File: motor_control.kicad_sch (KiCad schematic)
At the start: 109 parts, among them J1 Conn_01x18_Pin, J2 Conn_01x18_Pin, J3 Conn_01x10_Pin

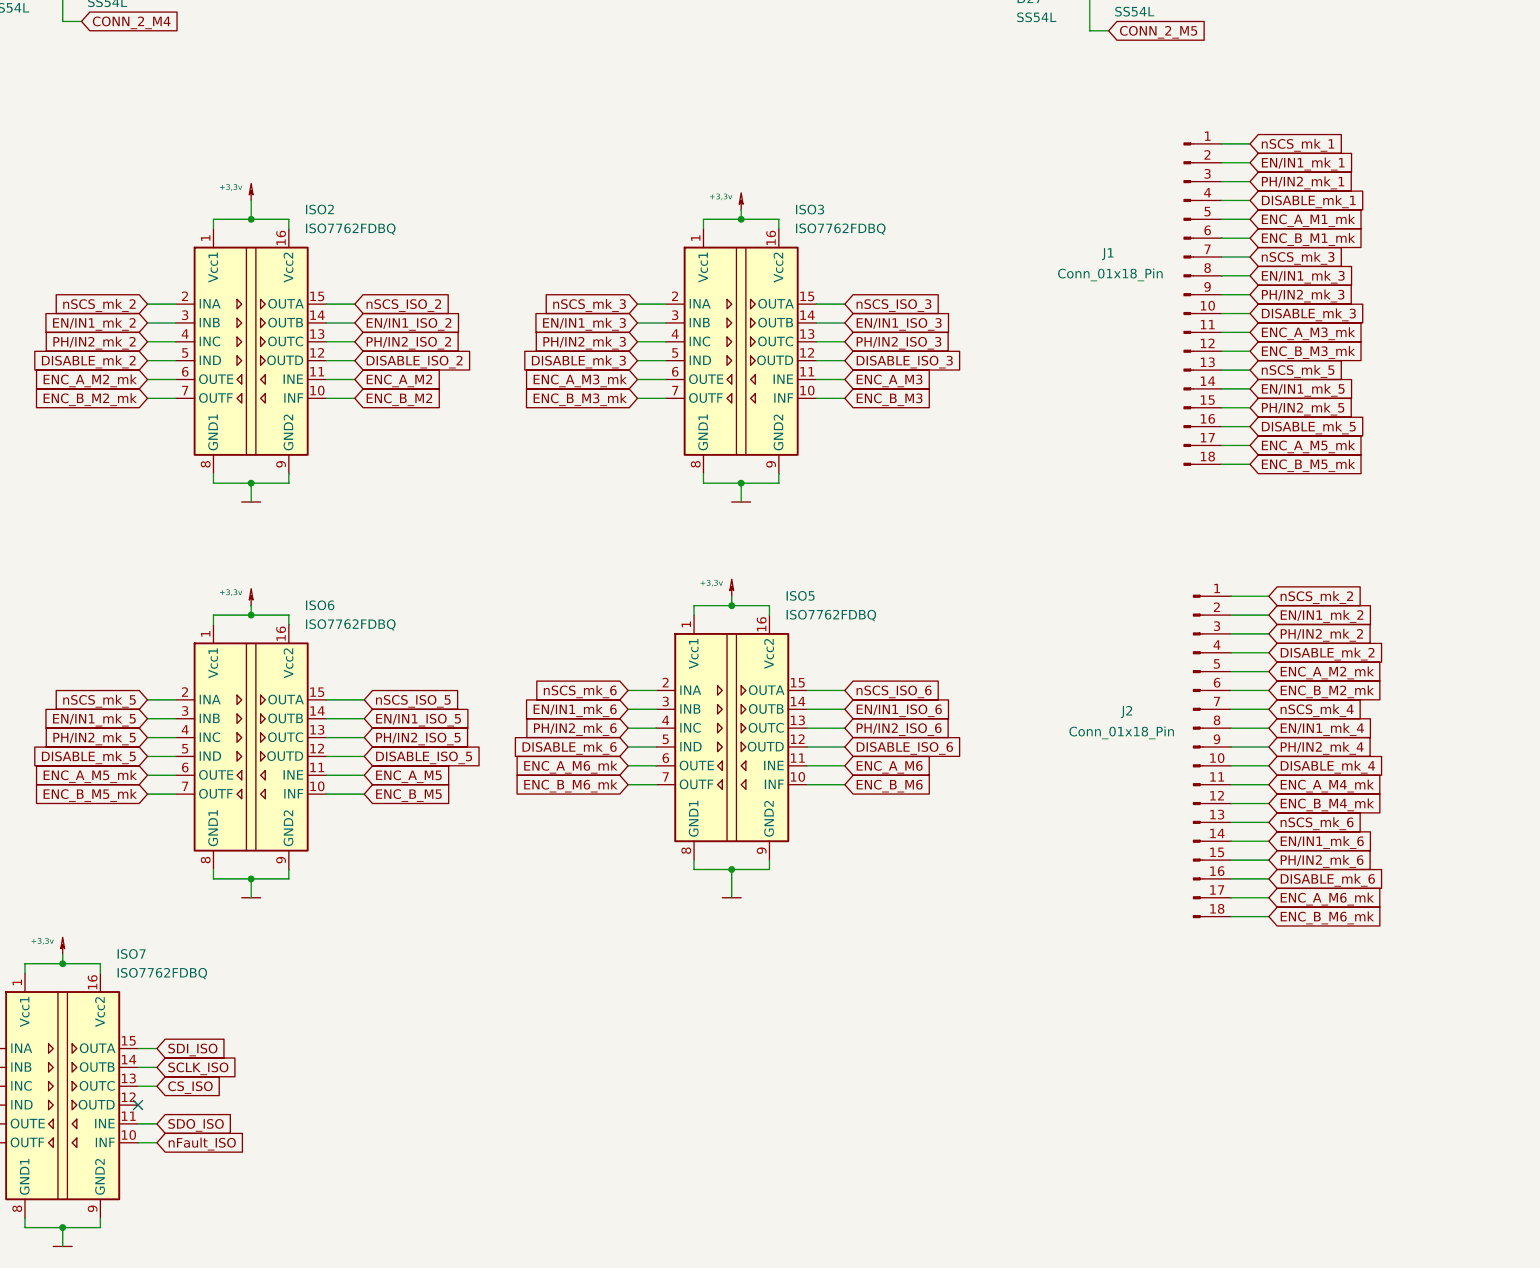
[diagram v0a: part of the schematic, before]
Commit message: I2C
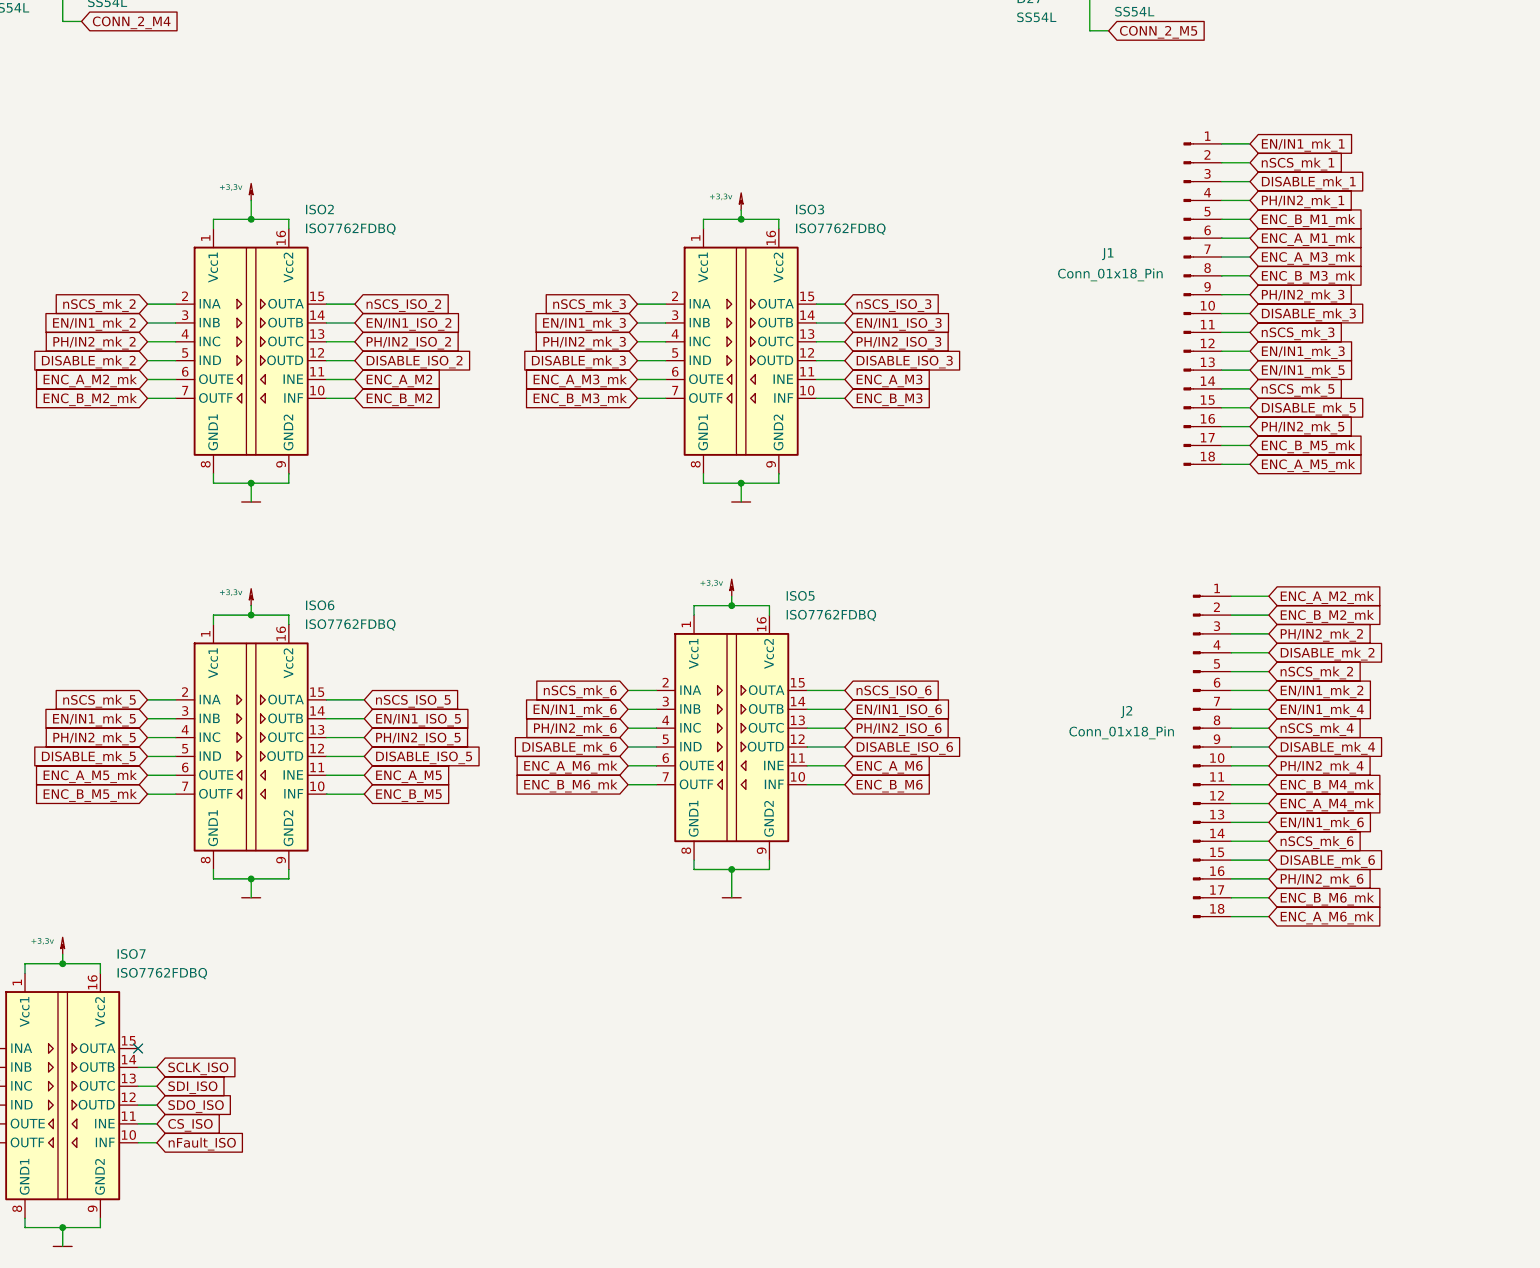
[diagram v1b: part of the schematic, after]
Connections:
- net CS_ISO: now also ISO7.11 (INE); no longer ISO7.13 (OUTC)
- net DISABLE_mk_1: now also J1.3 (Pin_3); no longer J1.4 (Pin_4)
- net DISABLE_mk_4: now also J2.9 (Pin_9); no longer J2.10 (Pin_10)
- net DISABLE_mk_5: now also J1.15 (Pin_15); no longer J1.16 (Pin_16)
- net DISABLE_mk_6: now also J2.15 (Pin_15); no longer J2.16 (Pin_16)
- net ENC_A_M1_mk: now also J1.6 (Pin_6); no longer J1.5 (Pin_5)
- net ENC_A_M2_mk: now also J2.1 (Pin_1); no longer J2.5 (Pin_5)
- net ENC_A_M3_mk: now also J1.7 (Pin_7); no longer J1.11 (Pin_11)
- net ENC_A_M4_mk: now also J2.12 (Pin_12); no longer J2.11 (Pin_11)
- net ENC_A_M5_mk: now also J1.18 (Pin_18); no longer J1.17 (Pin_17)
- net ENC_A_M6_mk: now also J2.18 (Pin_18); no longer J2.17 (Pin_17)
- net ENC_B_M1_mk: now also J1.5 (Pin_5); no longer J1.6 (Pin_6)
- net ENC_B_M2_mk: now also J2.2 (Pin_2); no longer J2.6 (Pin_6)
- net ENC_B_M3_mk: now also J1.8 (Pin_8); no longer J1.12 (Pin_12)
- net ENC_B_M4_mk: now also J2.11 (Pin_11); no longer J2.12 (Pin_12)
- net ENC_B_M5_mk: now also J1.17 (Pin_17); no longer J1.18 (Pin_18)
- net ENC_B_M6_mk: now also J2.17 (Pin_17); no longer J2.18 (Pin_18)
- net EN/IN1_mk_1: now also J1.1 (Pin_1); no longer J1.2 (Pin_2)
- net EN/IN1_mk_2: now also J2.6 (Pin_6); no longer J2.2 (Pin_2)
- net EN/IN1_mk_3: now also J1.12 (Pin_12); no longer J1.8 (Pin_8)
- net EN/IN1_mk_4: now also J2.7 (Pin_7); no longer J2.8 (Pin_8)
- net EN/IN1_mk_5: now also J1.13 (Pin_13); no longer J1.14 (Pin_14)
- net EN/IN1_mk_6: now also J2.13 (Pin_13); no longer J2.14 (Pin_14)
- net PH/IN2_mk_1: now also J1.4 (Pin_4); no longer J1.3 (Pin_3)
- net PH/IN2_mk_4: now also J2.10 (Pin_10); no longer J2.9 (Pin_9)
- net PH/IN2_mk_5: now also J1.16 (Pin_16); no longer J1.15 (Pin_15)
- net PH/IN2_mk_6: now also J2.16 (Pin_16); no longer J2.15 (Pin_15)
- net SDI_ISO: now also ISO7.13 (OUTC); no longer ISO7.15 (OUTA)
- net SDO_ISO: now also ISO7.12 (OUTD); no longer ISO7.11 (INE)
- net nSCS_mk_1: now also J1.2 (Pin_2); no longer J1.1 (Pin_1)
- net nSCS_mk_2: now also J2.5 (Pin_5); no longer J2.1 (Pin_1)
- net nSCS_mk_3: now also J1.11 (Pin_11); no longer J1.7 (Pin_7)
- net nSCS_mk_4: now also J2.8 (Pin_8); no longer J2.7 (Pin_7)
- net nSCS_mk_5: now also J1.14 (Pin_14); no longer J1.13 (Pin_13)
- net nSCS_mk_6: now also J2.14 (Pin_14); no longer J2.13 (Pin_13)

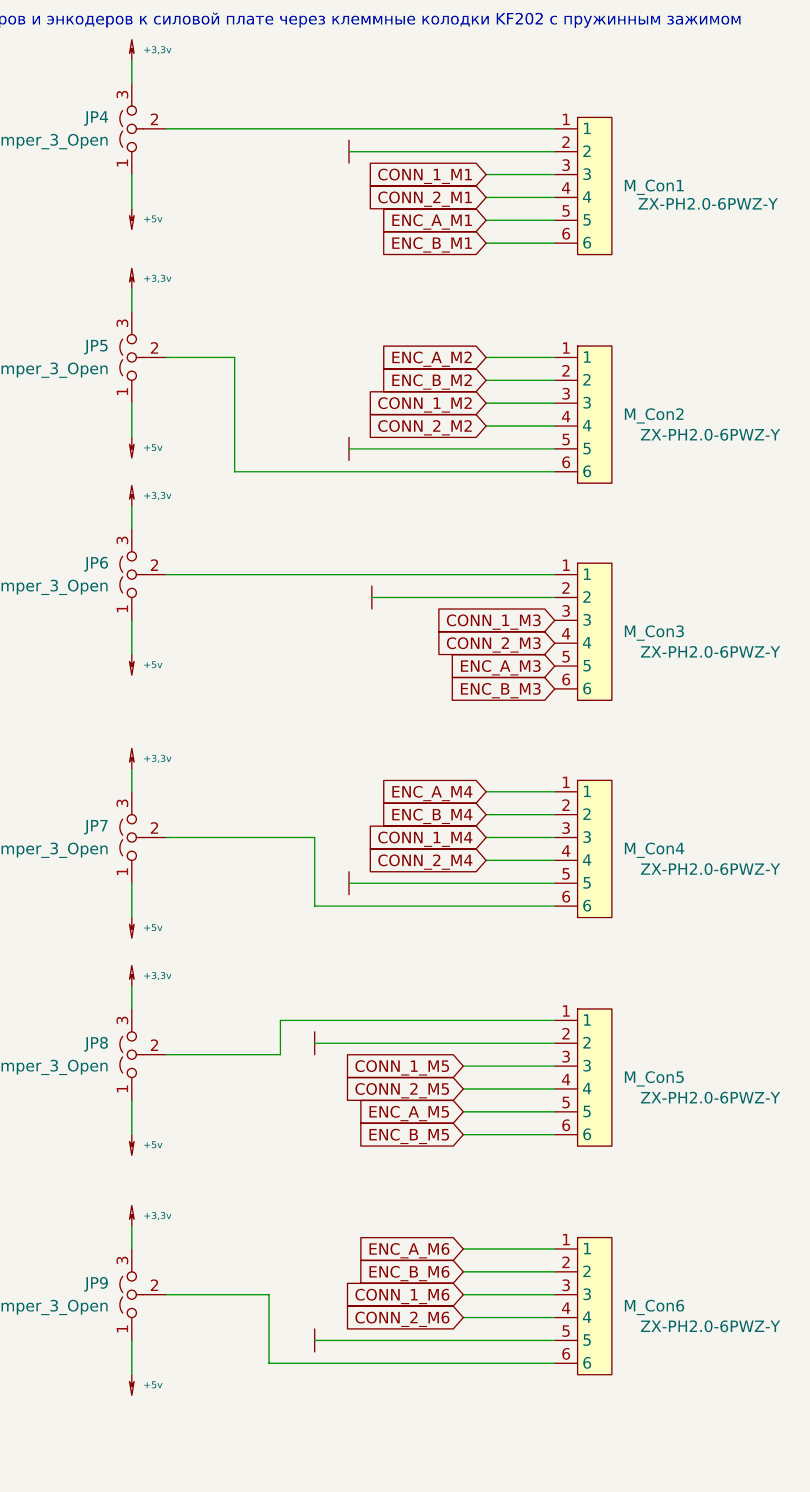
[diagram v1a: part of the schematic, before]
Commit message: 3v3MK
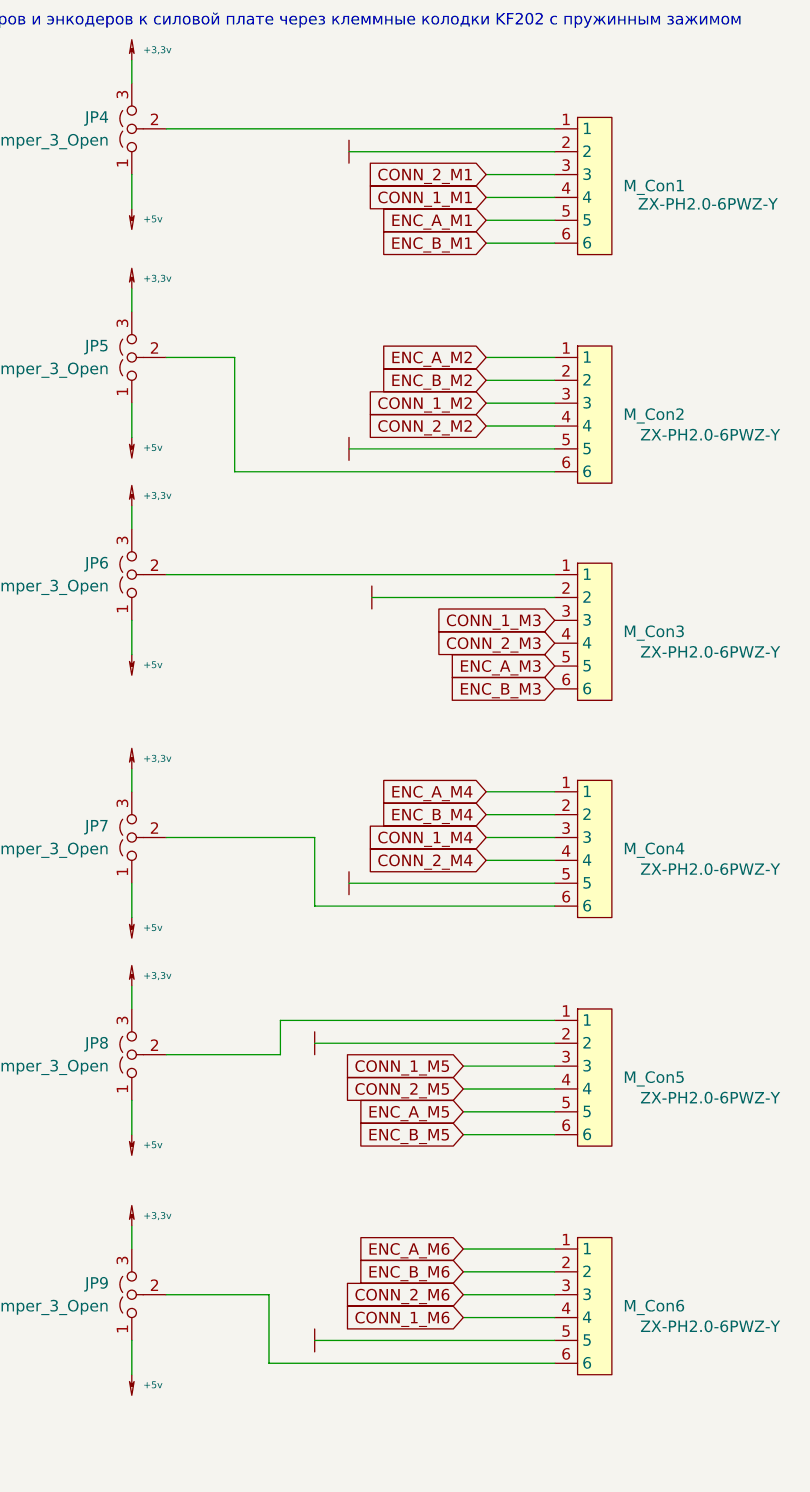
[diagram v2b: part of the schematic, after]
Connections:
- net CONN_1_M1: now also M_Con1.4; no longer M_Con1.3
- net CONN_1_M6: now also M_Con6.4; no longer M_Con6.3
- net CONN_2_M1: now also M_Con1.3; no longer M_Con1.4
- net CONN_2_M6: now also M_Con6.3; no longer M_Con6.4
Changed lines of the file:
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@@
 	(wire
 		(pts
+			(xy 538.48 31.75) (xy 546.1 31.75)
+		)
+		(stroke
+			(width 0)
+			(type default)
+		)
+	)
+	(wire
+		(pts
 			(xy 473.71 186.69) (xy 473.71 187.96)
 		)
@@
 	(wire
 		(pts
+			(xy 538.48 34.29) (xy 546.1 34.29)
+		)
+		(stroke
+			(width 0)
+			(type default)
+		)
+	)
+	(wire
+		(pts
 			(xy 347.98 54.61) (xy 349.25 54.61)
 		)
@@
 	(wire
 		(pts
-			(xy 535.94 156.21) (xy 546.1 156.21)
-		)
-		(stroke
-			(width 0)
-			(type default)
-		)
-	)
-	(wire
-		(pts
 			(xy 356.87 106.68) (xy 359.41 106.68)
 		)
@@
 	(wire
 		(pts
-			(xy 535.94 158.75) (xy 546.1 158.75)
-		)
-		(stroke
-			(width 0)
-			(type default)
-		)
-	)
-	(wire
-		(pts
 			(xy 515.62 129.54) (xy 515.62 125.73)
 		)
@@
 	(wire
 		(pts
-			(xy 538.48 31.75) (xy 546.1 31.75)
-		)
-		(stroke
-			(width 0)
-			(type default)
-		)
-	)
-	(wire
-		(pts
 			(xy 383.54 64.77) (xy 386.08 64.77)
 		)
@@
 	(wire
 		(pts
+			(xy 535.94 156.21) (xy 546.1 156.21)
+		)
+		(stroke
+			(width 0)
+			(type default)
+		)
+	)
+	(wire
+		(pts
 			(xy 260.35 189.23) (xy 256.54 189.23)
 		)
@@
 	(wire
 		(pts
+			(xy 535.94 158.75) (xy 546.1 158.75)
+		)
+		(stroke
+			(width 0)
+			(type default)
+		)
+	)
+	(wire
+		(pts
 			(xy 424.18 213.36) (xy 425.45 213.36)
 		)
@@
 	(wire
 		(pts
-			(xy 538.48 34.29) (xy 546.1 34.29)
-		)
-		(stroke
-			(width 0)
-			(type default)
-		)
-	)
-	(wire
-		(pts
 			(xy 113.03 293.37) (xy 110.49 293.37)
 		)
@@
 	(global_label "CONN_1_M6"
 		(shape input)
-		(at 535.94 156.21 180)
+		(at 535.94 158.75 180)
 		(effects
 			(font
@@
 		)
 		(property "Intersheetrefs" "${INTERSHEET_REFS}"
-			(at 535.94 156.21 0)
+			(at 535.94 158.75 0)
 			(hide yes)
 			(show_name no)
@@
 	(global_label "CONN_2_M6"
 		(shape input)
-		(at 535.94 158.75 180)
+		(at 535.94 156.21 180)
 		(effects
 			(font
@@
 		)
 		(property "Intersheetrefs" "${INTERSHEET_REFS}"
-			(at 535.94 158.75 0)
+			(at 535.94 156.21 0)
 			(hide yes)
 			(show_name no)
@@
 	(global_label "CONN_2_M1"
 		(shape input)
-		(at 538.48 34.29 180)
+		(at 538.48 31.75 180)
 		(effects
 			(font
@@
 		)
 		(property "Intersheetrefs" "${INTERSHEET_REFS}"
-			(at 538.48 34.29 0)
+			(at 538.48 31.75 0)
 			(hide yes)
 			(show_name no)
@@
 	(global_label "CONN_1_M1"
 		(shape input)
-		(at 538.48 31.75 180)
+		(at 538.48 34.29 180)
 		(effects
 			(font
@@
 		)
 		(property "Intersheetrefs" "${INTERSHEET_REFS}"
-			(at 538.48 31.75 0)
+			(at 538.48 34.29 0)
 			(hide yes)
 			(show_name no)
